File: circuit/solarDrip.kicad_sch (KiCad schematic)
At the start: 22 parts, among them J1 DCDC_01x03_Socket, J2 MPPT_01x04_Pin, J3 solar_panel, J4 battery, J5 soil_moisture, J6 water_level, J7 pump, P1 USB_C_Plug_USB2.0, Q1 2N7002E, Q2 2N7002E, Q3 FDN340P, U1 ESP32-C3-WROOM-02

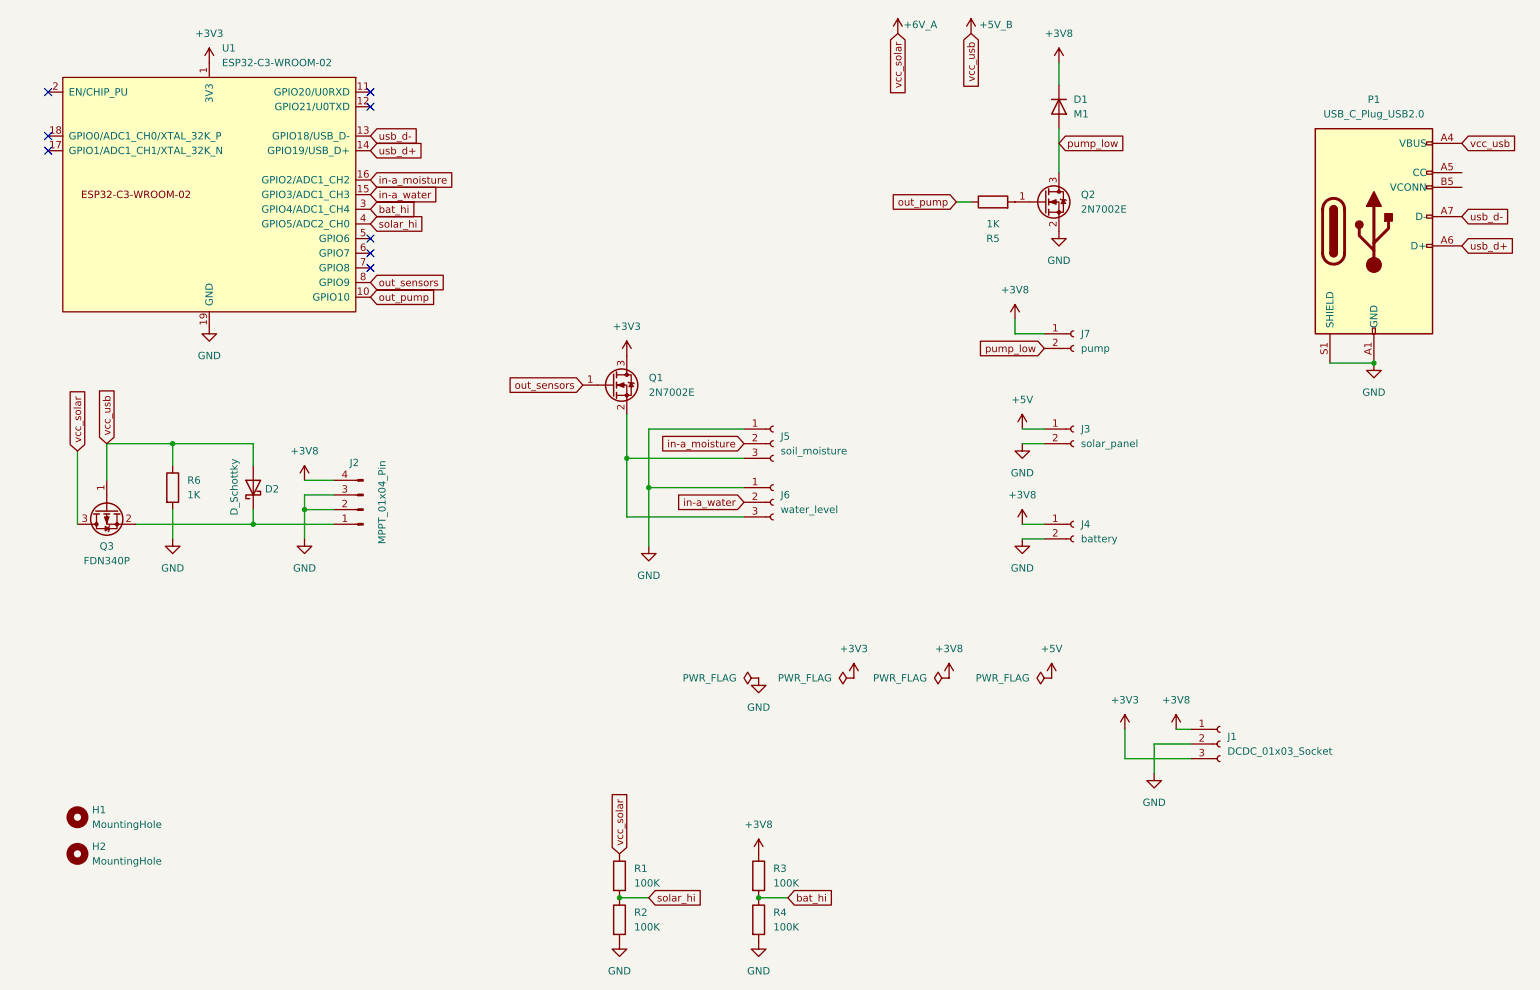
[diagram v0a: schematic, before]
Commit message: cleanup and annotations
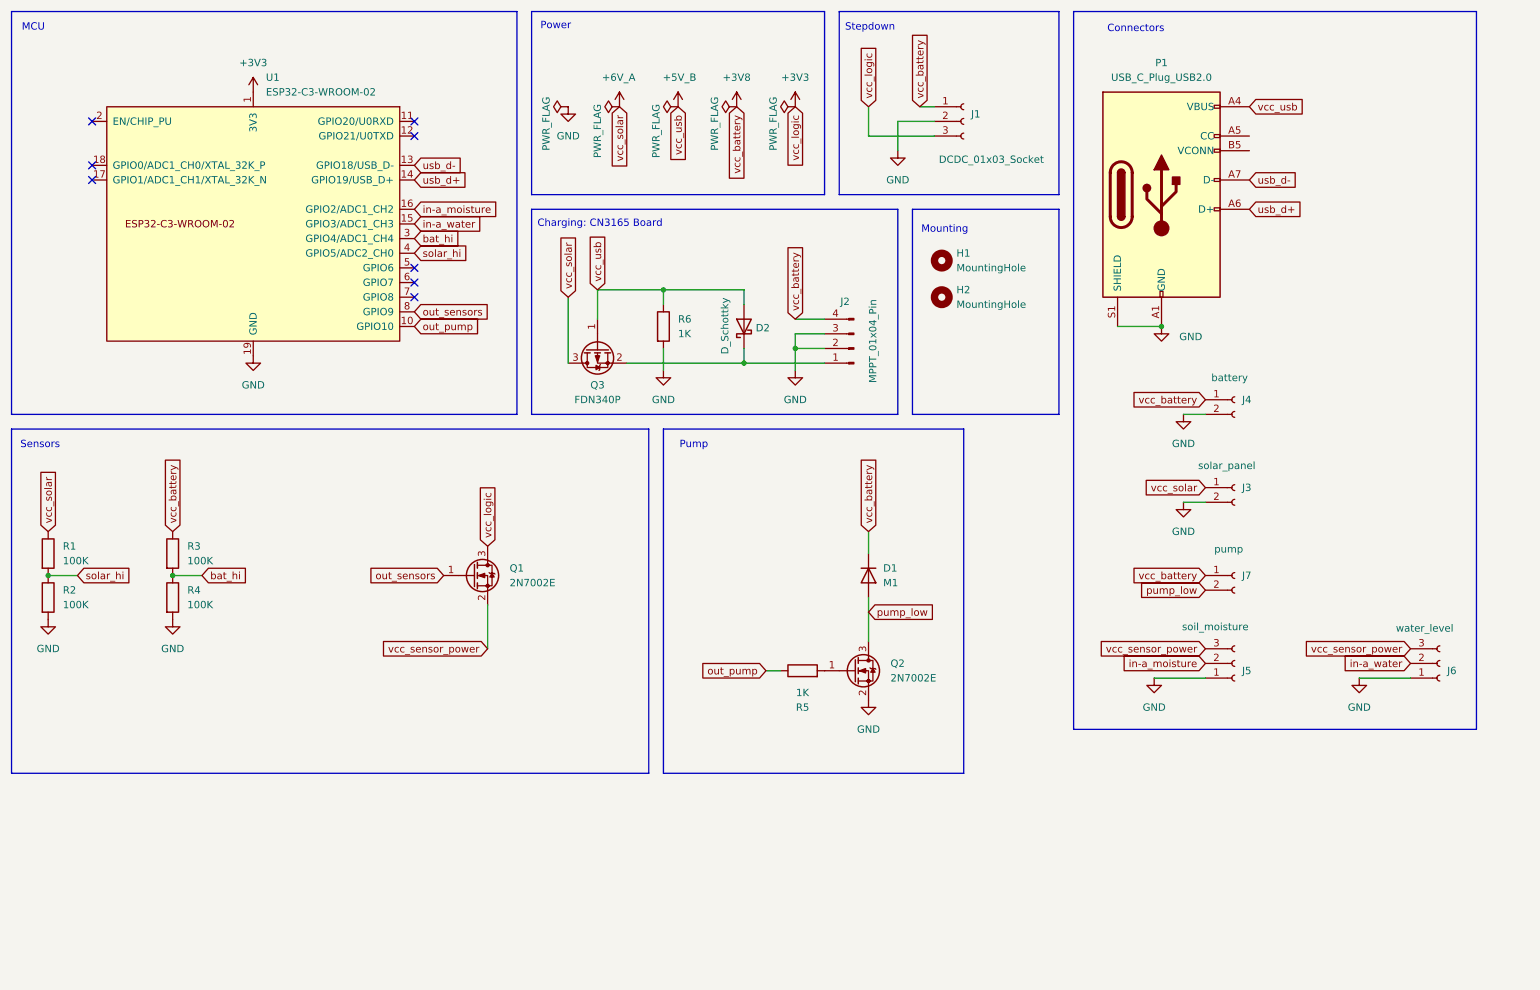
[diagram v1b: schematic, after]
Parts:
- P1: footprint (none) -> Connector_USB:USB_C_Plug_Molex_105444
- R6: footprint (none) -> Resistor_SMD:R_0402_1005Metric_Pad0.72x0.64mm_HandSolder
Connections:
- net +5V is gone; now on net +6V_A: J3.1 (Pin_1)
- net vcc_sensor_power: now reaches J5.3 (Pin_3), J6.3 (Pin_3), Q1.2 (S)
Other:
- note added: "Charging: CN3165 Board"
- note added: "Connectors"
- note added: "MCU"
- note added: "Mounting"
- note added: "Power"
- note added: "Pump"
- note added: "Sensors"
- note added: "Stepdown"
- moved on the sheet: D1, D2, H1, H2, J1, J2, J4, J5, J6, J7, P1, Q1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
